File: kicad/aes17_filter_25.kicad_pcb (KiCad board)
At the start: 2 copper layers, 193 x 92.6 mm, 38 parts, among them J1 NC3FAAH, J2 NC3MAAH, J3 Conn_01x01_Pin, J4 Conn_01x01_Pin, SW1 SW_DPST, SW2 SW_DPDT_x2

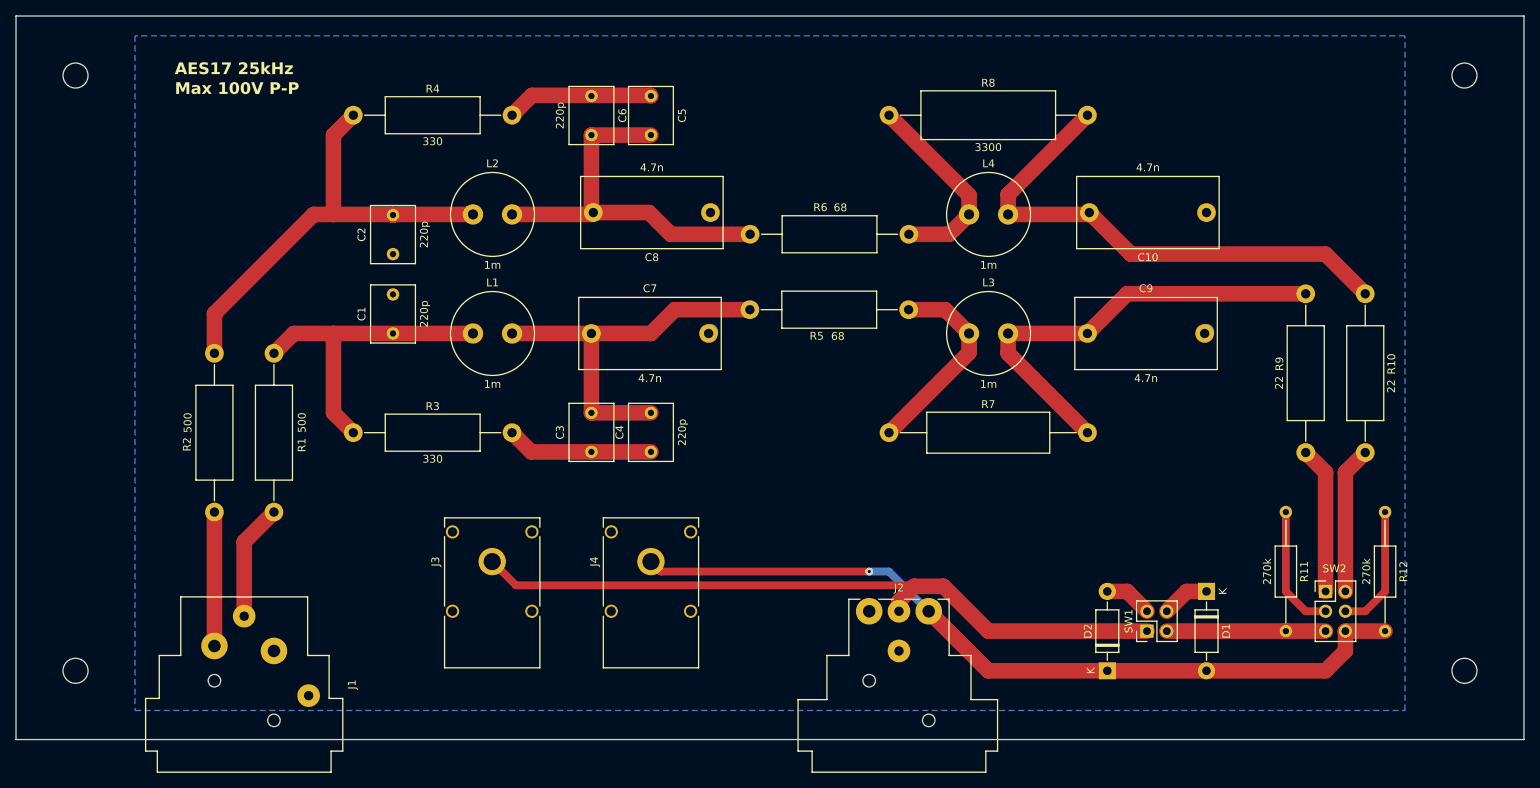
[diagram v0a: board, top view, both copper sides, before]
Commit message: Readme updated
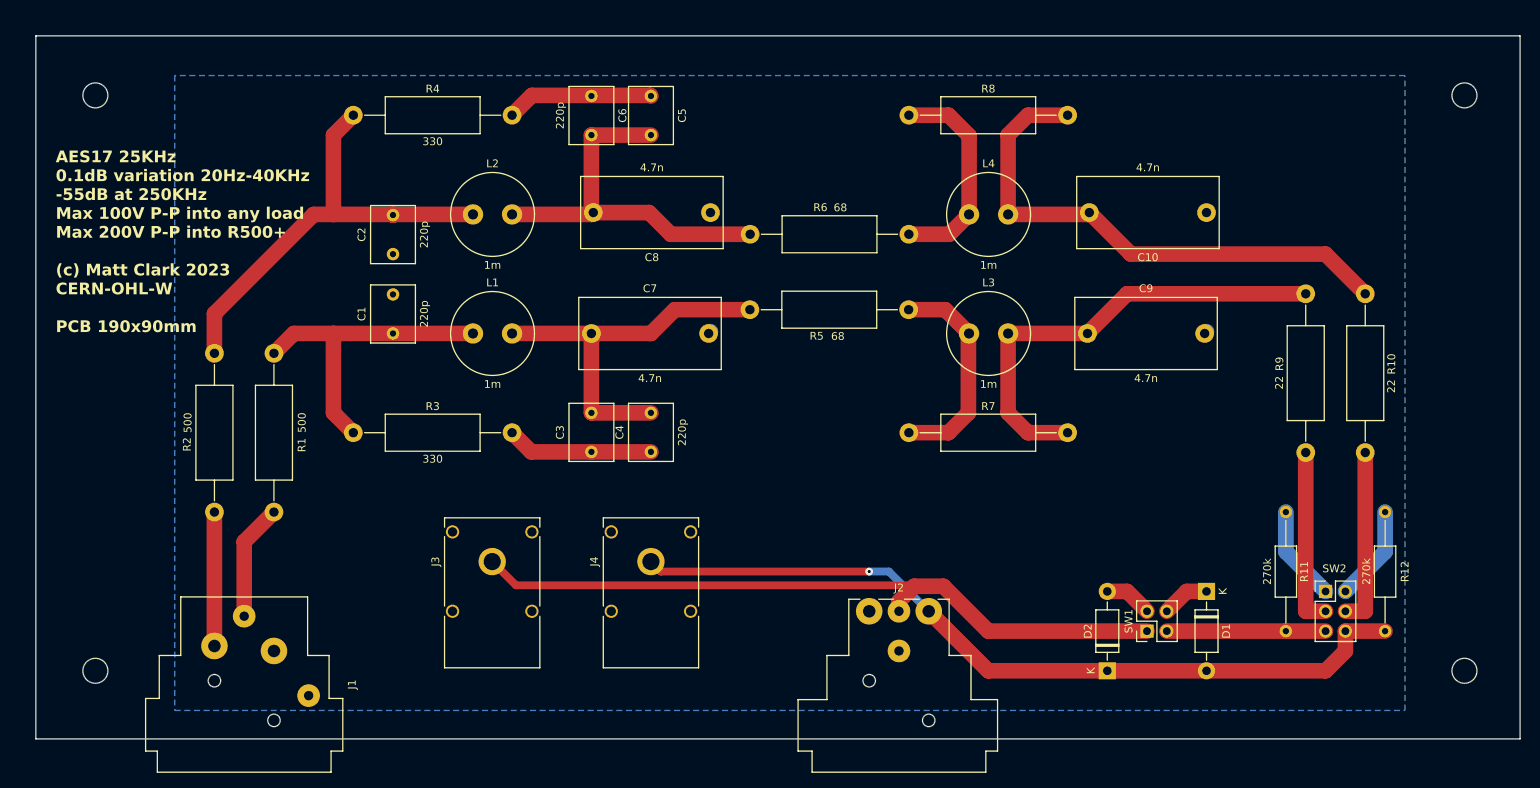
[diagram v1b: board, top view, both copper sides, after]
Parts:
- J1: value NC3FAAH -> NC3FAAH2
- R7: footprint Resistor_THT:R_Axial_DIN0516_L15.5mm_D5.0mm_P25.40mm_Horizontal -> Resistor_THT:R_Axial_DIN0414_L11.9mm_D4.5mm_P20.32mm_Horizontal
- R8: footprint Resistor_THT:R_Axial_DIN0617_L17.0mm_D6.0mm_P25.40mm_Horizontal -> Resistor_THT:R_Axial_DIN0414_L11.9mm_D4.5mm_P20.32mm_Horizontal
- moved H1 3.59 mm to (58.4, 55.9)
- moved H2 2.54 mm to (233.7, 55.9)
- moved H3 2.54 mm to (58.4, 129.5)
- moved R7 2.54 mm to (162.6, 99.1)
- moved R8 2.54 mm to (162.6, 58.4)
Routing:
- net Net-(SW2B-B): track 18.8 -> 22.9 mm
- net Net-(SW2A-B): track 18.8 -> 22.9 mm
- net Net-(SW2B-C): track 16.3 -> 12.3 mm
- net Net-(SW2A-C): track 16.3 -> 12.3 mm
- net Net-(C10-Pad2): track 67.0 -> 69.0 mm
- net Net-(L3-Pad1): track 25.9 -> 27.9 mm
- net Net-(L4-Pad1): track 25.7 -> 27.6 mm
- net Net-(C9-Pad1): track 57.1 -> 59.0 mm
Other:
- board size 193 x 92.6 mm -> 190 x 90 mm
- board text added: "AES17 25KHz 0.1dB variation 20Hz-40KHz -55dB at 250KHz Max 100V P-P into any load Max 200V P-P into R500+ (c) Matt Clark 2023 CERN-OHL-W PCB 190x90mm"
- board text removed: "AES17 25kHz"
- board text removed: "Max 100V P-P"
